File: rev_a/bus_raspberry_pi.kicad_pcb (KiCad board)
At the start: 2 copper layers, 100 x 50 mm, 51 parts, among them J1 TERMINATE_JUMPER, J2 LED_JUMPER, Q1 FQP47P06, SW1 MJTP1243, U1 74x05, U2 MCP2562, U3 74X08, U4 ATMEGA324_DIP40, X1 16MHz, X2 OSHW_LOGO

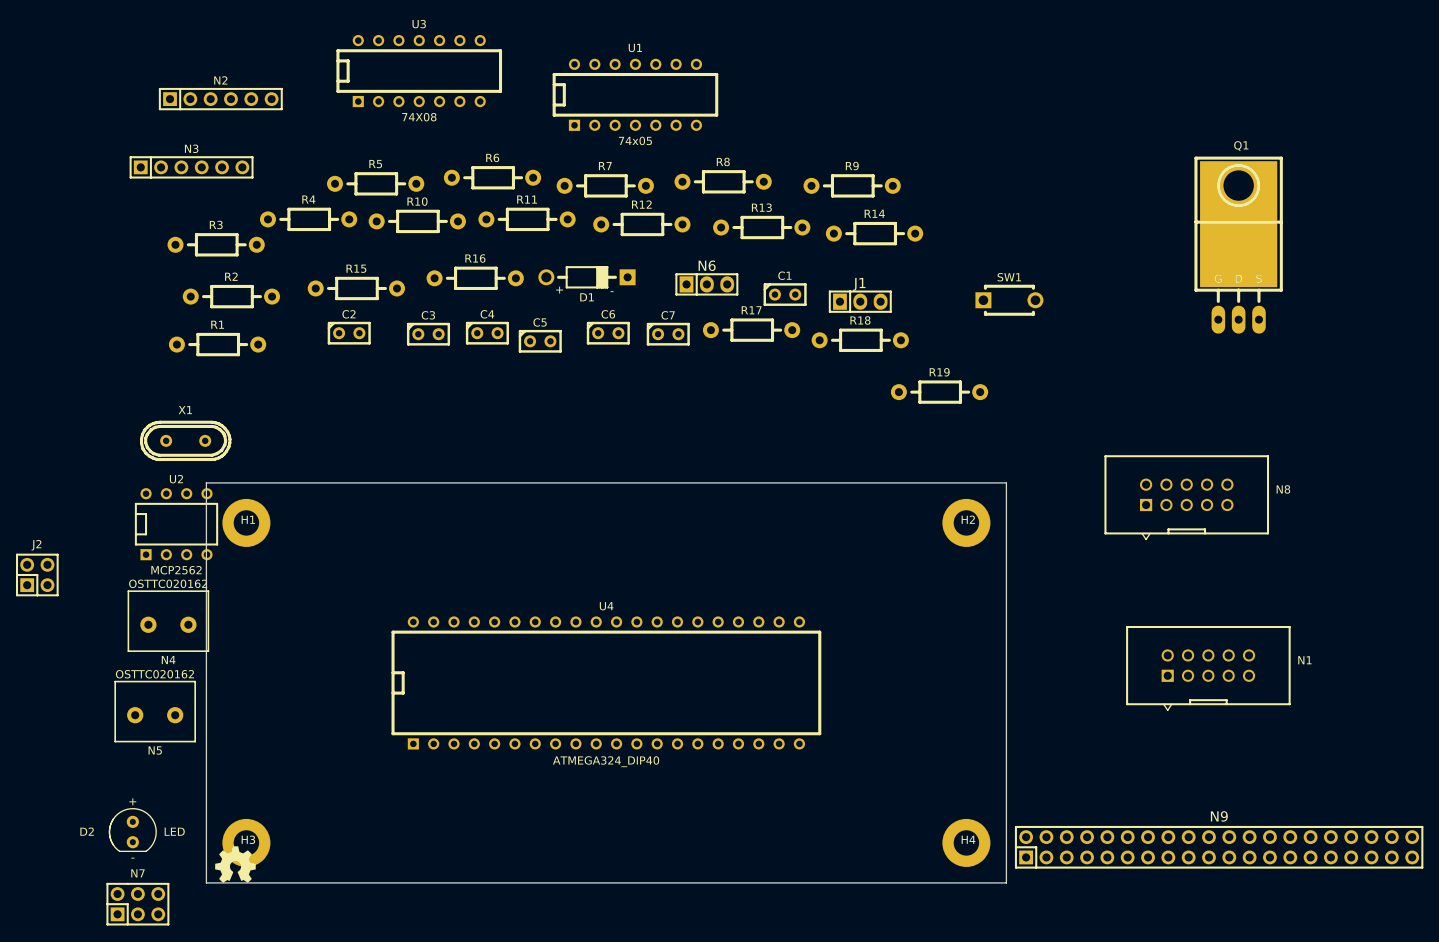
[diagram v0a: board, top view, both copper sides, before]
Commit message: Layed out PCB.
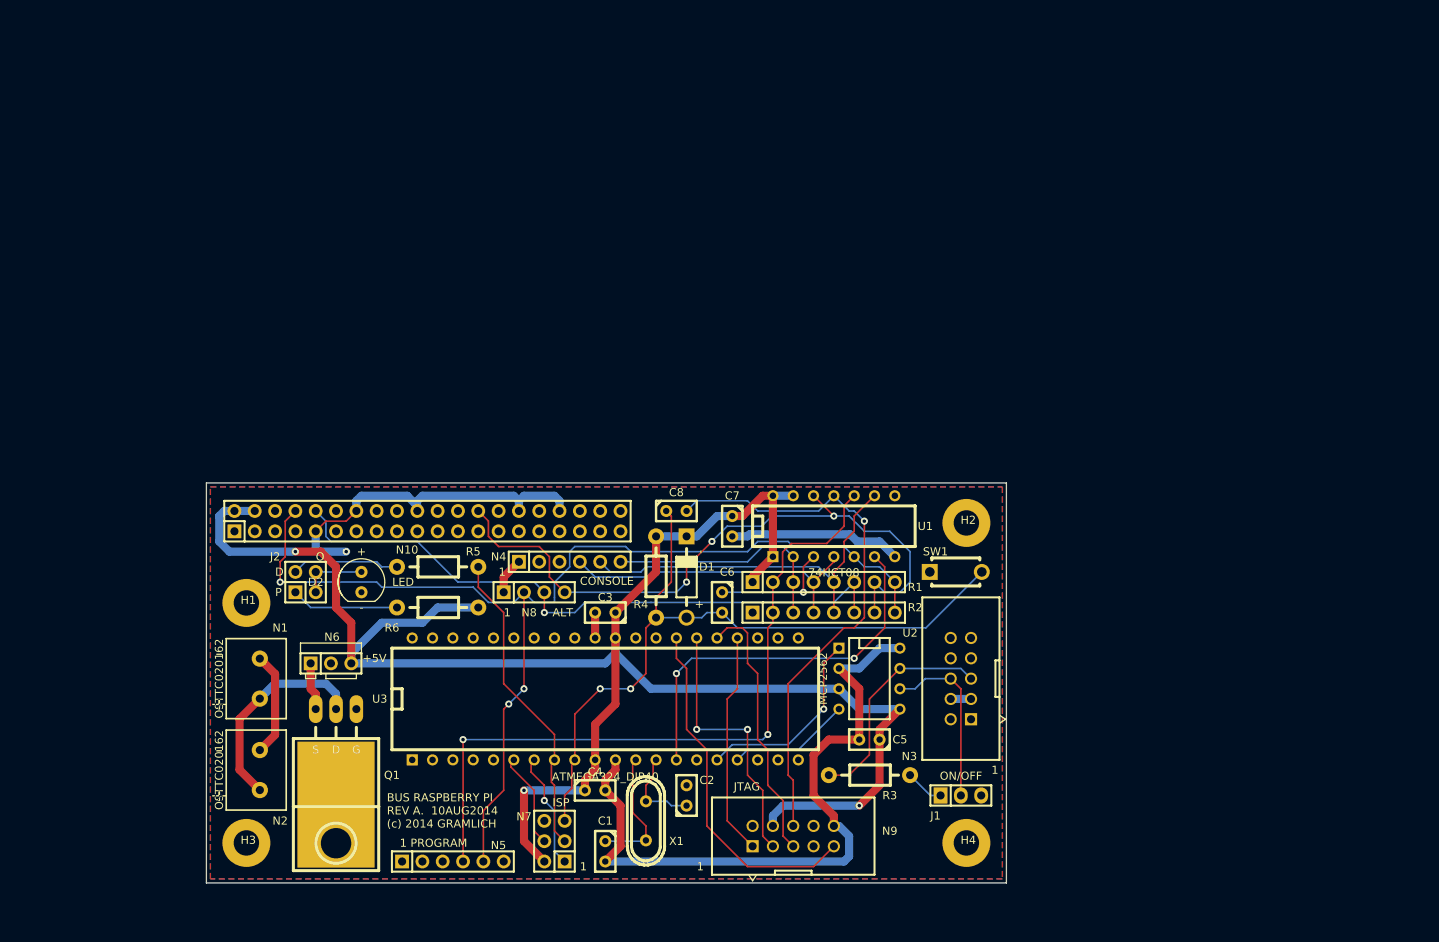
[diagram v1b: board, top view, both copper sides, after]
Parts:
- removed R10, R9: 10K, Bus_Raspberry_Pi_Rev_A:Resistor_Horizontal__400
- removed R11, R13, R16, R7: 22K 1%, Bus_Raspberry_Pi_Rev_A:Resistor_Horizontal__400
- removed R12, R14, R17, R8: 33K 1%, Bus_Raspberry_Pi_Rev_A:Resistor_Horizontal__400
- removed R15: 100K, Bus_Raspberry_Pi_Rev_A:Resistor_Horizontal__400
- removed R18, R19: 470, Bus_Raspberry_Pi_Rev_A:Resistor_Horizontal__400
- removed U4: ATMEGA324_DIP40, Bus_Raspberry_Pi_Rev_A:DIP-40__600
- added C8: .1uF, Bus_Raspberry_Pi_Rev_A:Capacitor3MMDiscRM2.5, F.Cu at (158.8, 103.5)
- added N10: RASPI_CONNECTOR_40, Bus_Raspberry_Pi_Rev_A:Pin_Header_Straight_2x20, F.Cu at (127.6, 104.8)
- N1: value BHR-10-HUA -> OSTTC020162; footprint Bus_Raspberry_Pi_Rev_A:Pin_Header_Straight_2x05_Shrouded -> Bus_Raspberry_Pi_Rev_A:5MM_TERMINAL_BLOCK_2_POS
- N2: value FTDI_HEADER -> OSTTC020162; footprint Bus_Raspberry_Pi_Rev_A:Pin_Header_Straight_1x06 -> Bus_Raspberry_Pi_Rev_A:5MM_TERMINAL_BLOCK_2_POS
- N3: value FTDI_HEADER -> BHR-10-HUA; footprint Bus_Raspberry_Pi_Rev_A:Pin_Header_Straight_1x06 -> Bus_Raspberry_Pi_Rev_A:Pin_Header_Straight_2x05_Shrouded
- N4, N5: value OSTTC020162 -> FTDI_HEADER; footprint Bus_Raspberry_Pi_Rev_A:5MM_TERMINAL_BLOCK_2_POS -> Bus_Raspberry_Pi_Rev_A:Pin_Header_Straight_1x06
- N6: footprint Bus_Raspberry_Pi_Rev_A:Pin_Header_Straight_1x03 -> Bus_Raspberry_Pi_Rev_A:OKI_DC_TO_DC_CONNECTOR
- N8: value BHR-10-HUA -> SERIAL_CONNECTOR; footprint Bus_Raspberry_Pi_Rev_A:Pin_Header_Straight_2x05_Shrouded -> Bus_Raspberry_Pi_Rev_A:Pin_Header_Straight_1x04
- N9: value RASPI_CONNECTOR_40 -> BHR-10-HUA; footprint Pin_Headers:Pin_Header_Straight_2x20 -> Bus_Raspberry_Pi_Rev_A:Pin_Header_Straight_2x05_Shrouded
- R1: value 22K 1% -> 22K; footprint Bus_Raspberry_Pi_Rev_A:Resistor_Horizontal__400 -> Bus_Raspberry_Pi_Rev_A:Pin_Header_Straight_1x08
- R2: value 33K 1% -> 33K; footprint Bus_Raspberry_Pi_Rev_A:Resistor_Horizontal__400 -> Bus_Raspberry_Pi_Rev_A:Pin_Header_Straight_1x08
- R4: value 100K -> 10K
- R5: value 22K 1% -> 470
- R6: value 33K 1% -> 470
- U1: value 74x05 -> 74HCT08
- U3: value 74X08 -> ATMEGA324_DIP40; footprint Bus_Raspberry_Pi_Rev_A:DIP-14__300 -> Bus_Raspberry_Pi_Rev_A:DIP-40__600
- X2: moved to B.Cu
- moved Q1 122.9 mm to (116.2, 128.3), turned to 180 degrees
- moved N1 118.6 mm to (106.7, 124.5), turned to 90 degrees
- moved N3 115.5 mm to (194.3, 124.5), turned to 90 degrees
- moved R3 105.2 mm to (182.9, 136.5)
- moved U2 88.7 mm to (182.9, 124.5), turned to 270 degrees
- moved N2 84.0 mm to (106.7, 135.9), turned to 90 degrees
- moved R2 83.9 mm to (177.2, 116.2)
- moved N8 82.5 mm to (141.0, 113.7)
- moved U3 81.9 mm to (149.9, 127.0)
- moved R1 81.4 mm to (177.2, 112.4)
- moved X1 74.6 mm to (154.9, 142.2), turned to 90 degrees
- moved C1 73.1 mm to (149.9, 146.1), turned to 270 degrees
- moved C2 71.5 mm to (160.0, 139.1), turned to 90 degrees
- moved N6 66.7 mm to (115.6, 122.6)
- moved C5 64.6 mm to (182.9, 132.1), turned to 180 degrees
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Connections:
- C3 pad 1: Net-(C3-Pad1) -> +5V
- C3 pad 2: /~RESET -> GND
- C6 pad 1: +5V -> Net-(C6-Pad1)
- C6 pad 2: GND -> /~RESET
- J1 pad 2: Net-(J1-Pad2) -> /CANL
- N1 pad 1: Net-(N1-Pad1) -> /BAT+
- N1 pad 2: Net-(N1-Pad2) -> GND
- N2 pad 1: GND -> /BAT+
- N2 pad 2: Net-(N2-Pad2) -> GND
- N3 pad 1: GND -> Net-(N3-Pad1)
- N3 pad 3: Net-(N3-Pad3) -> GND
- N3 pad 4: Net-(N3-Pad4) -> GND
- N3 pad 5: Net-(N3-Pad5) -> /CANH
- N3 pad 6: Net-(N3-Pad6) -> /CANL
- N4 pad 1: Net-(N4-Pad1) -> GND
- N4 pad 2: GND -> Net-(N4-Pad2)
- N5 pad 1: Net-(N4-Pad1) -> GND
- N5 pad 2: GND -> Net-(N5-Pad2)
- N8 pad 1: /TCK -> GND
- N8 pad 2: GND -> Net-(N10-Pad8)
- N8 pad 3: /TDO -> Net-(N10-Pad10)
- N8 pad 4: +5V -> Net-(N10-Pad26)
- N9 pad 1: Net-(N9-Pad1) -> /TCK
- N9 pad 10: Net-(N9-Pad10) -> GND
- N9 pad 2: +5V -> GND
- N9 pad 3: Net-(N9-Pad3) -> /TDO
- N9 pad 5: Net-(N9-Pad5) -> /TMS
- N9 pad 6: Net-(N9-Pad6) -> Net-(C8-Pad2)
- N9 pad 8: Net-(N3-Pad5) -> Net-(N9-Pad8)
- N9 pad 9: GND -> /TDI
- Q1 pad D: Net-(N4-Pad1) -> /BAT+
- R1 pad 1: Net-(N3-Pad4) -> +5V
- R1 pad 2: +5V -> Net-(N5-Pad4)
- R2 pad 2: Net-(N3-Pad4) -> Net-(N5-Pad4)
- R3 pad 1: Net-(N1-Pad5) -> /CANH
- R4 pad 1: Net-(R4-Pad1) -> /~RESET
- R5 pad 1: Net-(N2-Pad6) -> Net-(J2-Pad2)
- R5 pad 2: +5V -> /SCK
- R6 pad 1: GND -> Net-(J2-Pad1)
- R6 pad 2: Net-(N2-Pad6) -> +5V
- U1 pad 1: Net-(N2-Pad6) -> +5V
- U1 pad 10: (no net) -> Net-(N5-Pad4)
- U1 pad 11: (no net) -> Net-(C8-Pad2)
- U1 pad 12: (no net) -> Net-(N10-Pad26)
- U1 pad 13: (no net) -> +5V
- U1 pad 2: Net-(R4-Pad1) -> Net-(N4-Pad6)
- U1 pad 3: Net-(R4-Pad1) -> Net-(C6-Pad1)
- U1 pad 4: Net-(C3-Pad1) -> Net-(N4-Pad4)
- U1 pad 5: Net-(N9-Pad26) -> Net-(N10-Pad8)
- U1 pad 6: /~RESET -> /RXD0
- U1 pad 8: (no net) -> Net-(R1-Pad1)
- U1 pad 9: (no net) -> Net-(N4-Pad5)
- U2 pad 6: Net-(J1-Pad2) -> /CANL
- U2 pad 7: Net-(N1-Pad5) -> /CANH
- U3 pad 1: Net-(N2-Pad4) -> Net-(U3-Pad1)
- U3 pad 10: (no net) -> +5V
- U3 pad 11: (no net) -> GND
- U3 pad 12: (no net) -> /XTAL2
- U3 pad 13: (no net) -> /XTAL1
- U3 pad 14: +5V -> /RXD0
- U3 pad 2: Net-(N3-Pad5) -> Net-(U3-Pad2)
- U3 pad 3: /RXD0 -> Net-(U3-Pad3)
- U3 pad 4: Net-(N2-Pad5) -> Net-(U3-Pad4)
- U3 pad 5: Net-(N3-Pad4) -> Net-(U3-Pad5)
- U3 pad 6: Net-(R13-Pad2) -> /MOSI
- U3 pad 7: GND -> /MISO
- U3 pad 8: (no net) -> /SCK
- U3 pad 9: (no net) -> /~RESET
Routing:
- net +5V: track 0.00 -> 240.9 mm, vias 0 -> 3
- net GND: track 0.00 -> 174.9 mm, vias 0 -> 1
- net Net-(N10-Pad8): track 0.00 -> 136.6 mm, vias 0 -> 3
- net /~RESET: track 0.00 -> 91.3 mm, vias 0 -> 2
- net Net-(N5-Pad4): track 0.00 -> 90.5 mm, vias 0 -> 2
- net Net-(N10-Pad26): track 0.00 -> 85.2 mm, vias 0 -> 3
- net Net-(N10-Pad10): track 0.00 -> 80.6 mm, vias 0 -> 1
- net Net-(C8-Pad2): track 0.00 -> 68.4 mm, vias 0 -> 1
- net /RXD0: track 0.00 -> 48.6 mm, vias 0 -> 2
- net Net-(N4-Pad5): track 0.00 -> 47.5 mm
- net /TDI: track 0.00 -> 44.1 mm
- net Net-(N4-Pad4): track 0.00 -> 39.5 mm
- net /SCK: track 0.00 -> 38.9 mm
- net /TDO: track 0.00 -> 33.7 mm, vias 0 -> 2
- net /TMS: track 0.00 -> 33.6 mm
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- added copper zone on B.Cu, net GND
- added copper zone on F.Cu, net GND
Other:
- net class Default: clearance 0.254 -> 0.2032; trace_width 0.254 -> 0.2032
- net class Power added: clearance 0.2032, trace_width 1.016, via_dia 0.889, via_drill 0.635
- rule trace_clearance: 0.254 -> 0.2032
- rule trace_min: 0.254 -> 0.2032
- board text added: "+"
- board text added: "+5V"
- board text added: "-"
- board text added: "1"
- board text added: "1 PROGRAM"
- board text added: "ALT"
- board text added: "BUS RASPBERRY PI REV A. 10AUG2014 (c) 2014 GRAMLICH"
- board text added: "CONSOLE"
- board text added: "D"
- board text added: "ISP"
- board text added: "JTAG"
- board text added: "O"
- board text added: "ON/OFF"
- board text added: "P"
- board text added: "hardware"
- board text added: "open source"
